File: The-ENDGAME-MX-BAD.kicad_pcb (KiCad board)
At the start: 2 copper layers, 76 parts, among them J2 Conn_01x02_Female, SW1 SW_Push, SW10 SW_Push, SW11 SW_Push, SW12 SW_Push, SW13 SW_Push, SW14 SW_Push, SW15 SW_Push, SW16 SW_Push, SW17 SW_Push, SW18 SW_Push, SW19 SW_Push, SW2 SW_Push, SW20 SW_Push, SW21 SW_Push, SW22 SW_Push, SW23 SW_Push, SW24 SW_Push, SW25 SW_Push, SW26 SW_Push, SW27 SW_Push, SW28 SW_Push, SW29 SW_Push, SW3 SW_Push, SW30 SW_Push, SW31 SW_Push, SW32 SW_Push, SW33 SW_Push, SW34 SW_Push, SW35 SW_Push, SW36 SW_Push, SW4 SW_Push, SW5 SW_Push, SW6 SW_Push, SW7 SW_Push, SW8 SW_Push, SW9 SW_Push, U1 ProMicro-kbd-34key

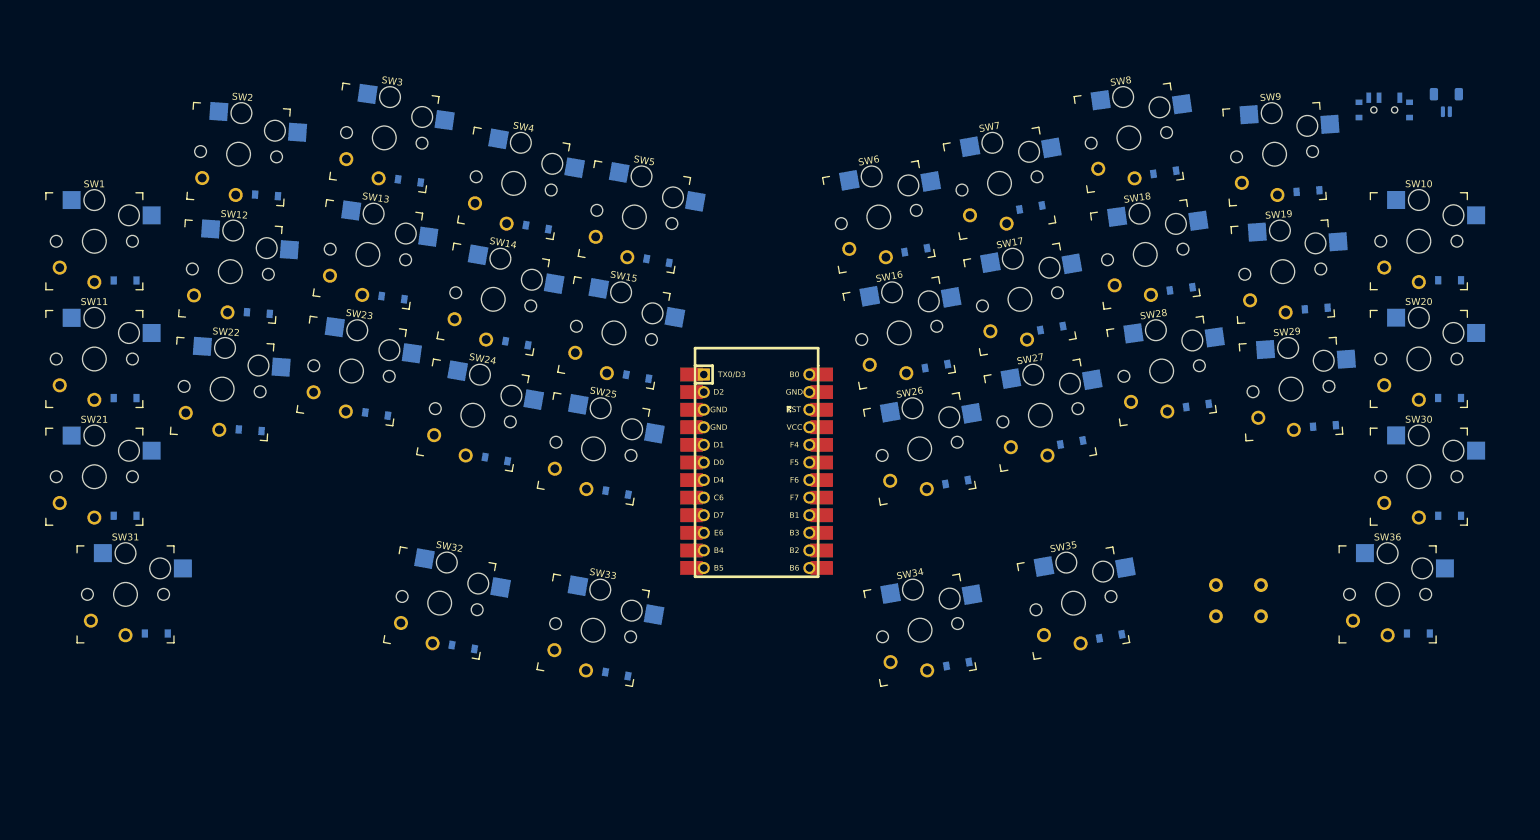
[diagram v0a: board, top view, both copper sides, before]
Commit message: pcb changes
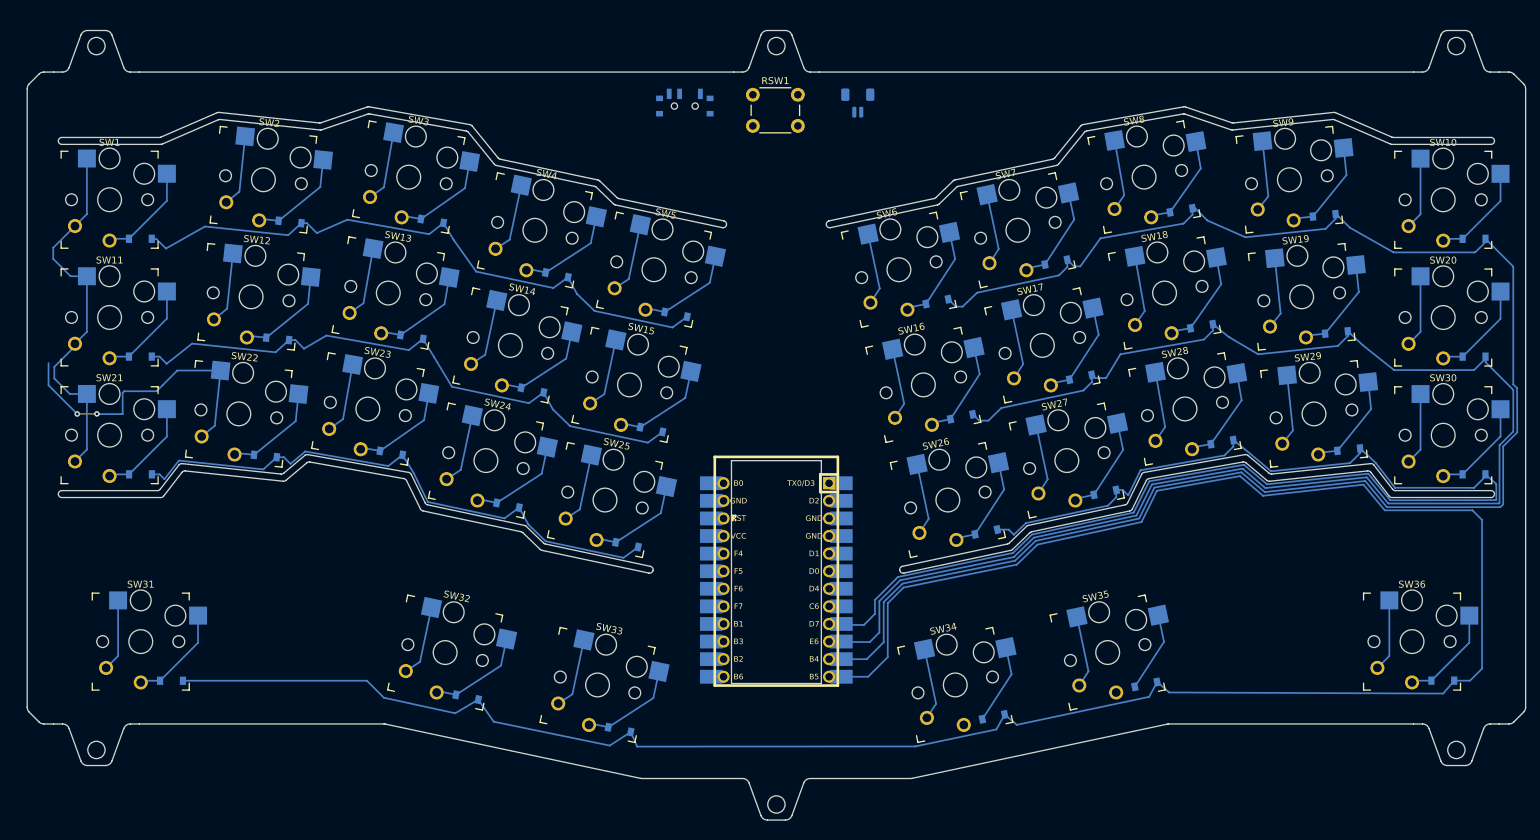
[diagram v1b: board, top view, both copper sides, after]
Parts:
- RSW1: moved to F.Cu
- U1: moved to B.Cu
- moved RSW1 102.0 mm to (144.0, 53.3), turned to 0 degrees
- moved SW_POWER1 101.0 mm to (134.2, 54.6)
- moved J2 85.0 mm to (159.1, 54.5)
- moved U1 16.0 mm to (147.4, 123.4)
- moved SW34 9.40 mm to (173.2, 138.5), turned to 12 degrees
- moved D34 9.21 mm to (178.7, 143.1), turned to -168 degrees
- moved D7 8.70 mm to (187.8, 77.5), turned to -168 degrees
- moved D27 8.68 mm to (194.9, 110.7), turned to -168 degrees
- moved SW35 8.67 mm to (195.2, 133.8), turned to 12 degrees
- moved D35 8.61 mm to (200.8, 138.4), turned to -168 degrees
- moved SW26 8.44 mm to (172.2, 111.8), turned to 12 degrees
- moved D26 8.37 mm to (177.7, 116.4), turned to -168 degrees
- moved SW16 8.27 mm to (168.6, 95.2), turned to 12 degrees
- moved D17 8.24 mm to (191.3, 94.1), turned to -168 degrees
- moved D16 8.18 mm to (174.1, 99.8), turned to -168 degrees
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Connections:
- D1 pad 1: col0 -> row0
- D10 pad 1: col0 -> row0
- D11 pad 1: col1 -> row1
- D12 pad 1: col1 -> row1
- D13 pad 1: col1 -> row1
- D14 pad 1: col1 -> row1
- D15 pad 1: col1 -> row1
- D16 pad 1: col1 -> row1
- D17 pad 1: col1 -> row1
- D18 pad 1: col1 -> row1
- D19 pad 1: col1 -> row1
- D2 pad 1: col0 -> row0
- D20 pad 1: col1 -> row1
- D21 pad 1: col2 -> row2
- D22 pad 1: col2 -> row2
- D23 pad 1: col2 -> row2
- D24 pad 1: col2 -> row2
- D25 pad 1: col2 -> row2
- D26 pad 1: col2 -> row2
- D27 pad 1: col2 -> row2
- D28 pad 1: col2 -> row2
- D29 pad 1: col2 -> row2
- D3 pad 1: col0 -> row0
- D30 pad 1: col2 -> row2
- D31 pad 1: col3 -> row3
- D32 pad 1: col3 -> row3
- D33 pad 1: col3 -> row3
- D34 pad 1: col3 -> row3
- D35 pad 1: col3 -> row3
- D36 pad 1: col3 -> row3
- D4 pad 1: col0 -> row0
- D5 pad 1: col0 -> row0
- D6 pad 1: col0 -> row0
- D7 pad 1: col0 -> row0
- D8 pad 1: col0 -> row0
- D9 pad 1: col0 -> row0
- SW1 pad 2: row0 -> col0
- SW11 pad 2: row0 -> col0
- SW12 pad 2: row1 -> col1
- SW13 pad 2: row2 -> col2
- SW14 pad 2: row3 -> col3
- SW15 pad 2: row4 -> col4
- SW16 pad 2: row5 -> col5
- SW17 pad 2: row6 -> col6
- SW18 pad 2: row7 -> col7
- SW19 pad 2: row8 -> col8
- SW2 pad 2: row1 -> col1
- SW21 pad 2: row0 -> col0
- SW22 pad 2: row1 -> col1
- SW23 pad 2: row2 -> col2
- SW24 pad 2: row3 -> col3
- SW25 pad 2: row4 -> col4
- SW26 pad 2: row5 -> col5
- SW27 pad 2: row6 -> col6
- SW28 pad 2: row7 -> col7
- SW29 pad 2: row8 -> col8
- SW3 pad 2: row2 -> col2
- SW31 pad 2: row0 -> col0
- SW32 pad 2: row3 -> col3
- SW33 pad 2: row4 -> col4
- SW34 pad 2: row5 -> col5
- SW35 pad 2: row6 -> col6
- SW4 pad 2: row3 -> col3
- SW5 pad 2: row4 -> col4
- SW6 pad 2: row5 -> col5
- SW7 pad 2: row6 -> col6
- SW8 pad 2: row7 -> col7
- SW9 pad 2: row8 -> col8
- U1 pad 11: row2 -> row0
- U1 pad 15: row9 -> unconnected-(U1-Pad15)
- U1 pad 16: row8 -> unconnected-(U1-Pad16)
- U1 pad 17: row7 -> unconnected-(U1-Pad17)
- U1 pad 18: row6 -> unconnected-(U1-Pad18)
- U1 pad 19: row5 -> unconnected-(U1-Pad19)
- U1 pad 20: row4 -> unconnected-(U1-Pad20)
- U1 pad 5: col0 -> unconnected-(U1-Pad5)
- U1 pad 6: col1 -> unconnected-(U1-Pad6)
- U1 pad 7: col2 -> unconnected-(U1-Pad7)
- U1 pad 8: col3 -> unconnected-(U1-Pad8)
- U1 pad 9: row0 -> row2
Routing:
- net row3: track 0.00 -> 331.5 mm
- net row0: track 0.00 -> 331.4 mm
- net row1: track 0.00 -> 304.7 mm
- net row2: track 0.00 -> 277.1 mm
- net col0: track 0.00 -> 66.0 mm
- net col1: track 0.00 -> 65.6 mm, vias 0 -> 2
- net col4: track 0.00 -> 41.9 mm
- net row9: track 0.00 -> 41.9 mm
- net col6: track 0.00 -> 41.9 mm
- net col3: track 0.00 -> 41.9 mm
- net col5: track 0.00 -> 41.9 mm
- net col8: track 0.00 -> 31.4 mm
- net col7: track 0.00 -> 31.4 mm
- net col2: track 0.00 -> 31.4 mm
- net Net-(D21-Pad2): track 0.00 -> 14.6 mm
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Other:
- board outline added: 216.4 x 114 mm

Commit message: soweit so gut ENDGAME outline und layout final
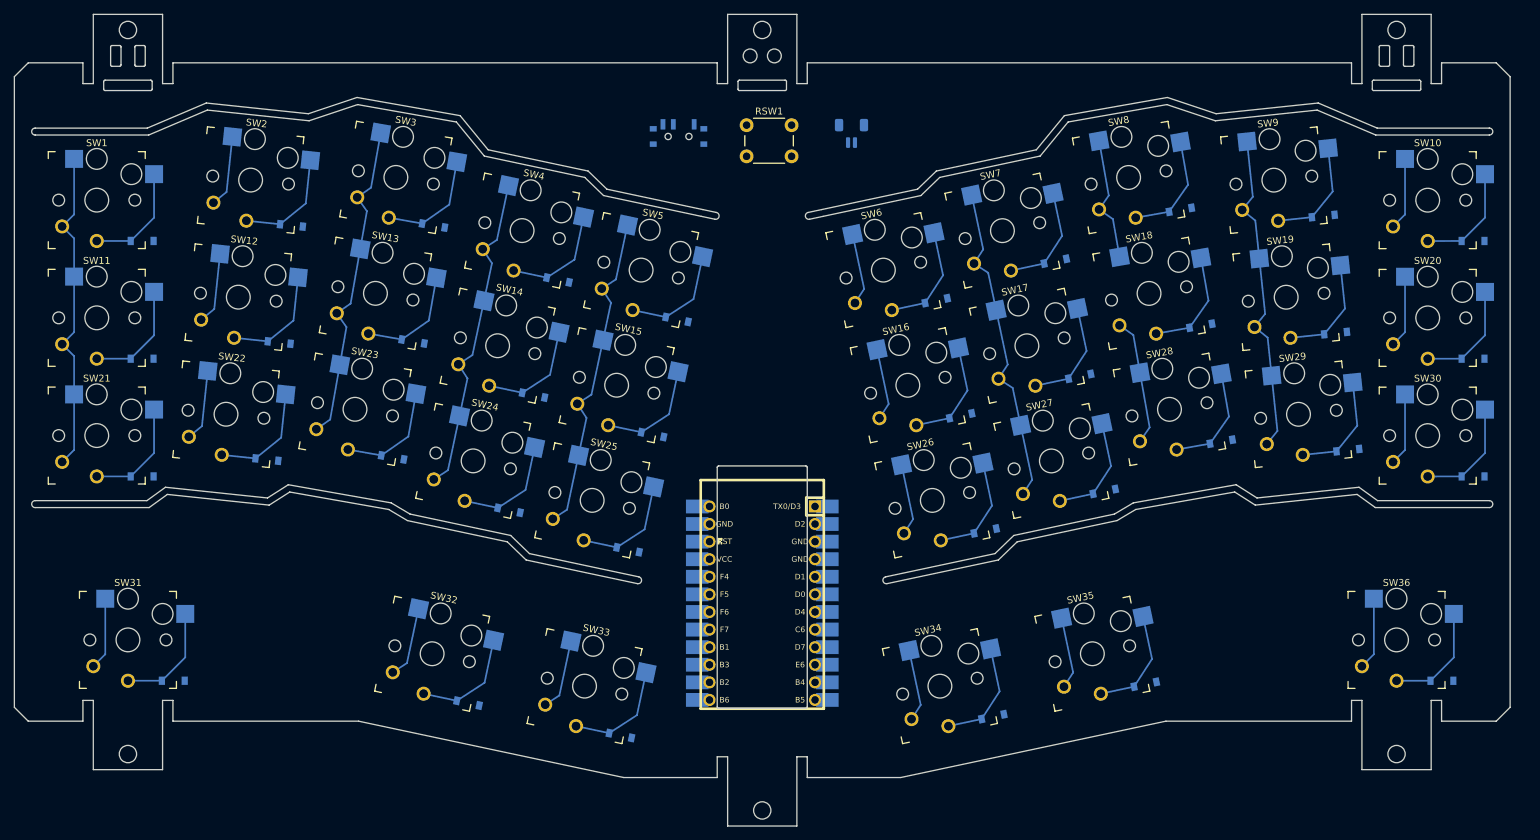
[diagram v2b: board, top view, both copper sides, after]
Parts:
- moved SW_POWER1 4.49 mm to (133.3, 59.0)
- moved RSW1 4.49 mm to (143.1, 57.7)
- moved J2 4.49 mm to (158.2, 58.9)
- moved U1 3.92 mm to (145.3, 126.7)
- moved SW36 2.25 mm to (236.9, 132.0)
- moved SW16 2.25 mm to (166.4, 95.2)
- moved SW26 2.25 mm to (169.9, 111.9)
- moved SW6 2.25 mm to (162.8, 78.6)
- moved SW20 2.24 mm to (241.4, 85.5)
- moved SW10 2.24 mm to (241.4, 68.5)
- moved SW30 2.24 mm to (241.4, 102.5)
- moved SW9 2.24 mm to (219.2, 65.6)
- moved SW29 2.24 mm to (222.8, 99.4)
- moved SW19 2.24 mm to (221.0, 82.5)
- moved SW8 2.24 mm to (198.3, 65.2)
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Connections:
- SW10 pad 2: row9 -> col9
- SW20 pad 2: row9 -> col9
- SW30 pad 2: row9 -> col9
- SW36 pad 2: row9 -> col9
- U1 pad 13: unconnected-(U1-Pad13) -> col0
- U1 pad 14: unconnected-(U1-Pad14) -> col1
- U1 pad 15: unconnected-(U1-Pad15) -> col2
- U1 pad 16: unconnected-(U1-Pad16) -> col3
- U1 pad 17: unconnected-(U1-Pad17) -> col4
- U1 pad 18: unconnected-(U1-Pad18) -> col5
- U1 pad 19: unconnected-(U1-Pad19) -> col6
- U1 pad 20: unconnected-(U1-Pad20) -> col7
- U1 pad 7: unconnected-(U1-Pad7) -> col9
- U1 pad 8: unconnected-(U1-Pad8) -> col8
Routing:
- net row3: track 331.5 -> 0.00 mm
- net row0: track 331.4 -> 0.00 mm
- net row1: track 304.7 -> 0.00 mm
- net row2: track 277.1 -> 0.00 mm
- net row9: track 41.9 -> 0.00 mm
- net col9: track 0.00 -> 41.9 mm
- net col1: track 65.6 -> 31.4 mm, vias 2 -> 0
- net col3: track 41.9 -> 57.8 mm
- net col2: track 31.4 -> 47.3 mm
- net col6: track 41.9 -> 57.8 mm
- net col4: track 41.9 -> 57.8 mm
- net col8: track 31.4 -> 47.3 mm
- net col0: track 66.0 -> 57.8 mm
- net col7: track 31.4 -> 36.9 mm
- net Net-(D35-Pad2): track 11.7 -> 15.9 mm
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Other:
- board size 216.4 x 114 mm -> 216 x 117.2 mm
